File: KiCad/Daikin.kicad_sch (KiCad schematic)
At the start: 20 parts, among them J1 SPOX, J2 Prog, Q1 PMF170XP,115, Q2 PMF250XNEX, U1 ESP32-PICO-MINI-02, U2 LMR16006+FB

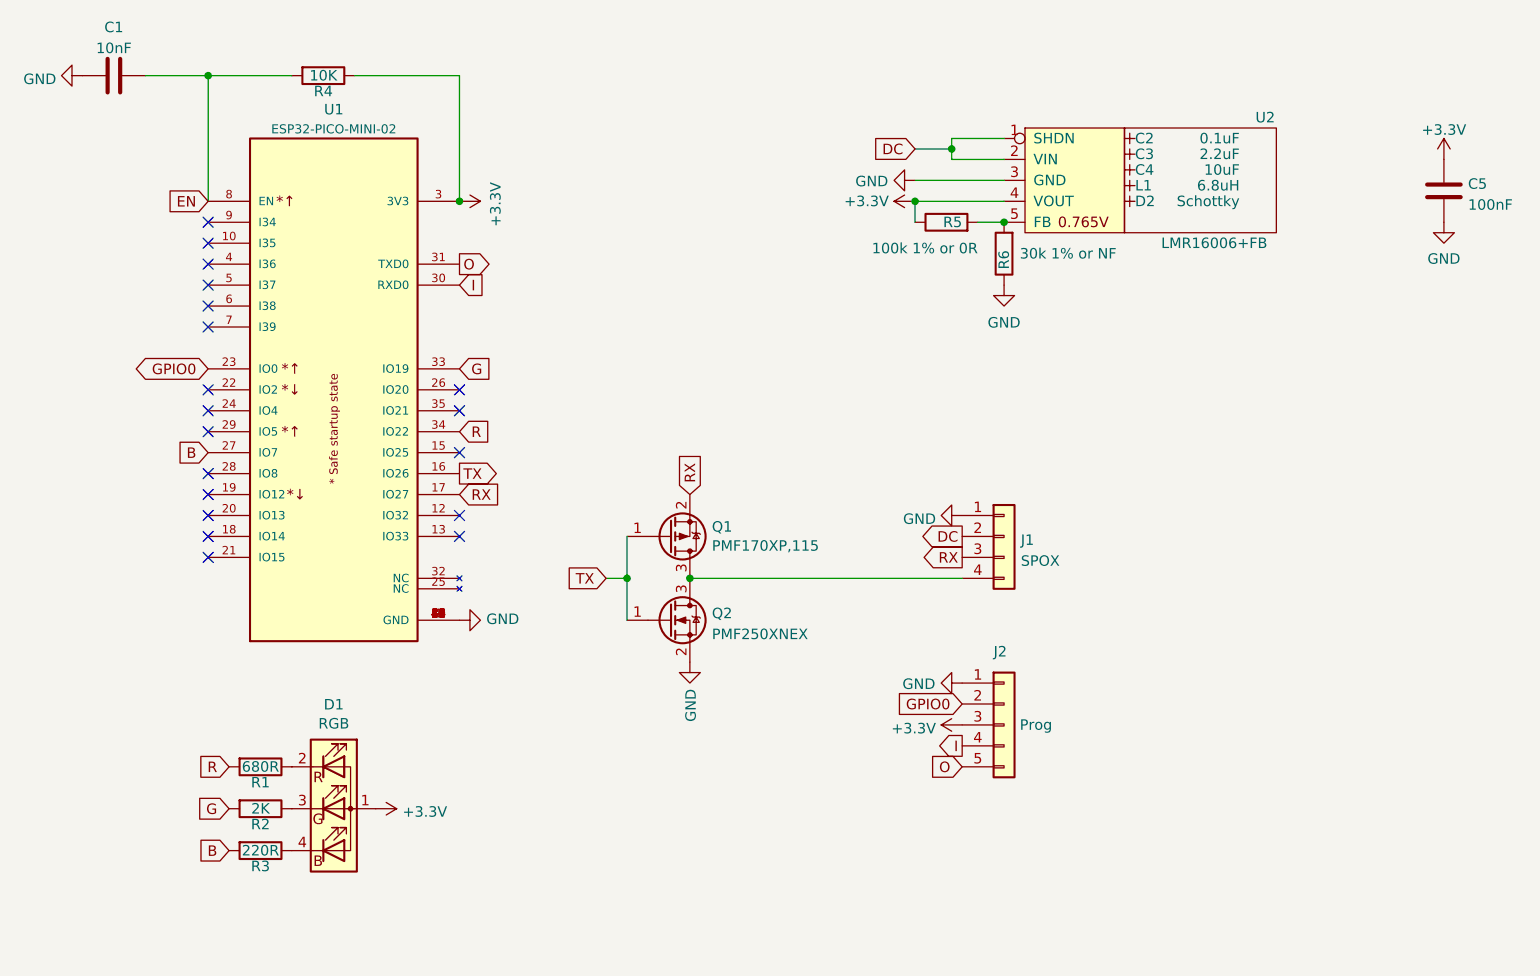
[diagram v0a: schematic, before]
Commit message: Started reverse engineering
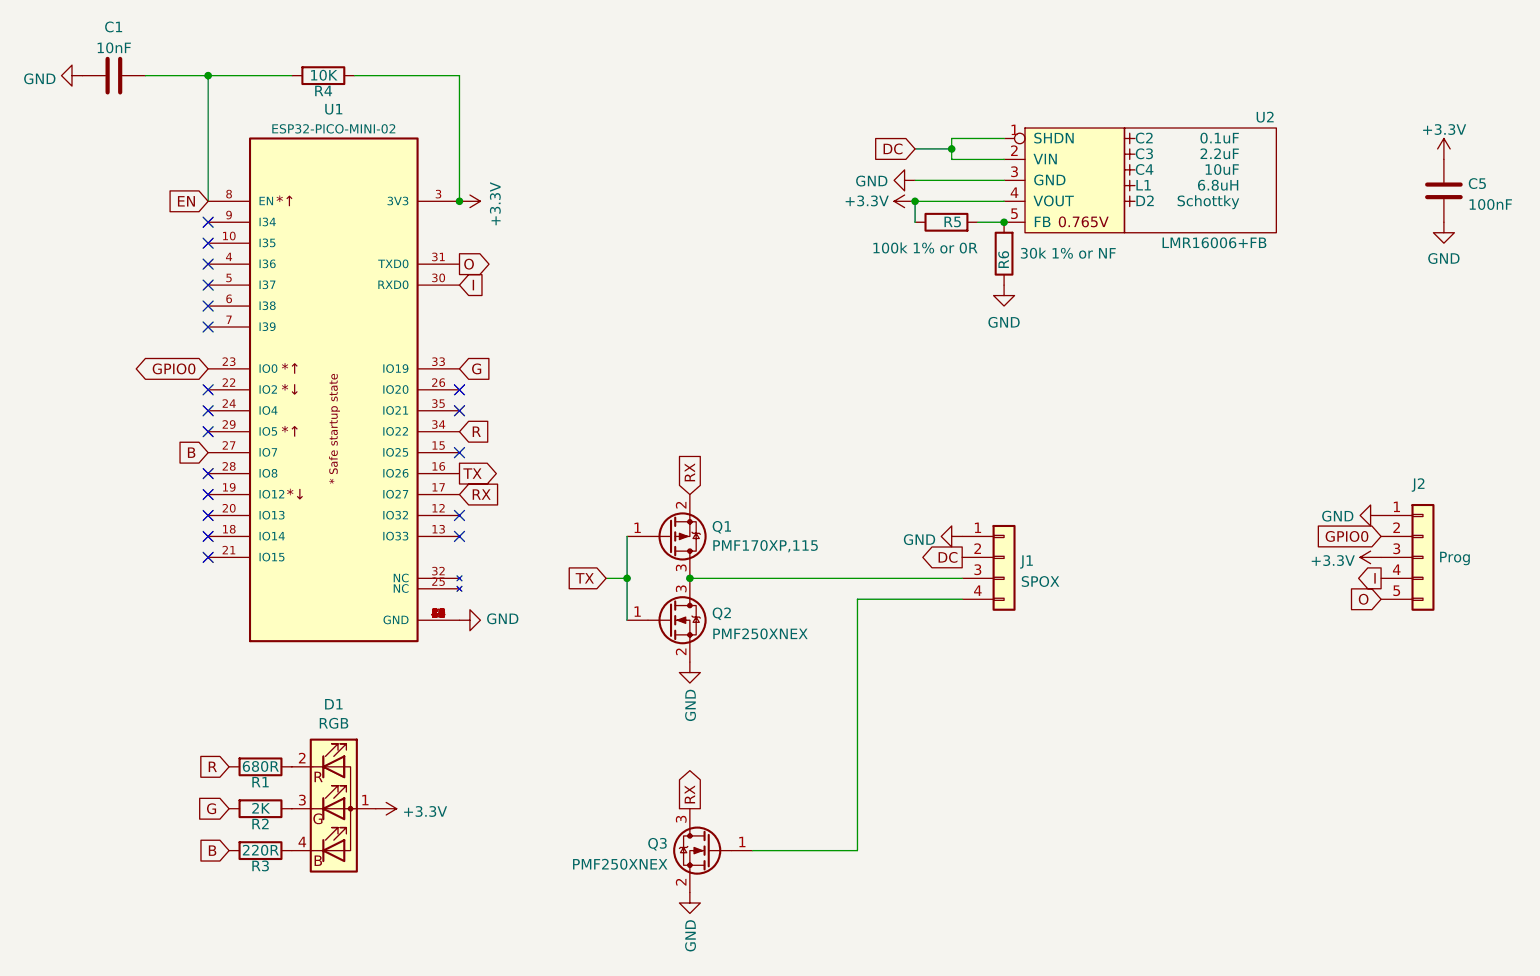
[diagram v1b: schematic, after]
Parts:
- added Q3: PMF250XNEX, Package_TO_SOT_SMD:SOT-323_SC-70, symbol RevK:NX7002AK
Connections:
- net GND: now also Q3.2 (S)
- net RX: now also Q3.3 (D); no longer J1.3 (Pin_3)
- net at Q1.3 (D), Q2.3 (D): now also J1.3 (Pin_3); no longer J1.4 (Pin_4)
- new net: J1.4 (Pin_4), Q3.1 (G)
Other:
- moved on the sheet: J1, J2
